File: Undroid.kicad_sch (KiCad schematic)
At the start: 41 parts

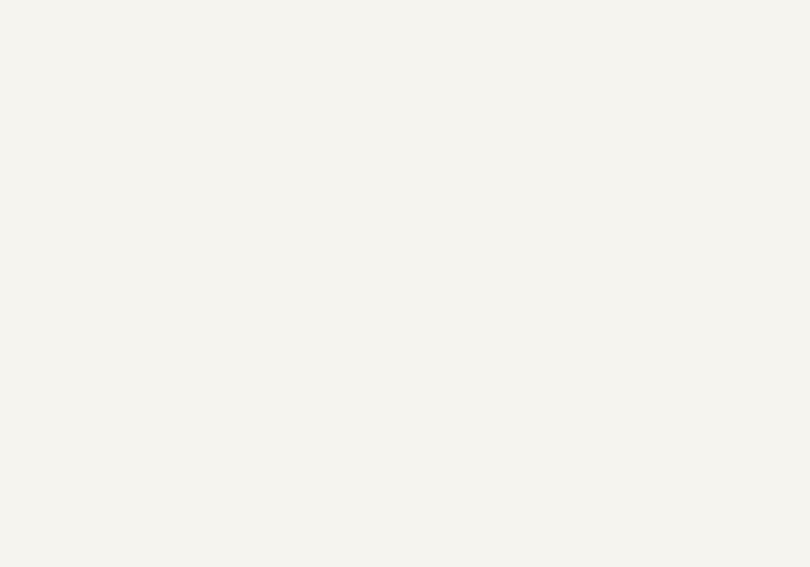
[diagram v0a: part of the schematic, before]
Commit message: Finishing routing.
Signed-off-by: Amlal EL Mahrouss <amlalelmahrouss@icloud.com>
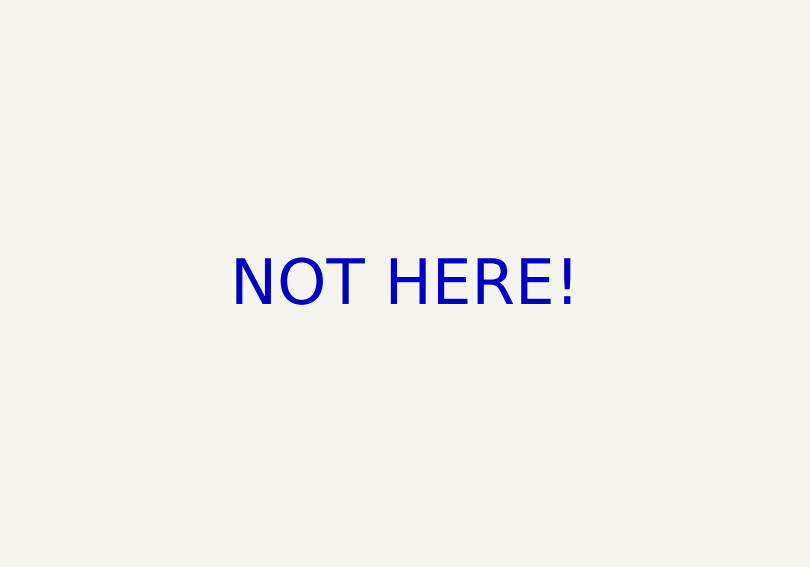
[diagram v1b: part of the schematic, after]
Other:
- note added: "NOT HERE!"
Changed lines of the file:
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@@
+		)
+	)
+	(text "NOT HERE!"
+		(exclude_from_sim yes)
+		(at 373.38 108.204 0)
+		(effects
+			(font
+				(size 5.08 5.08)
+			)
 		)
 	)
